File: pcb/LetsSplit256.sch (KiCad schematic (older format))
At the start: 62 parts, among them J1 AudioJack3_Ground, U1 ProMicro

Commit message: Add footprints for switch and pro micro
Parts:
- DL11, DL12, DL13, DL14, DL15, DL21, DL22, DL23, DL24, DL25, DL31, DL32, DL33, DL34, DL35, DL41, DL42, DL43, DL44, DL45, DL51, DL52, DL53, DL54, DL55, DL61, DL62, DL63, DL64, DL65: footprint Diodes_THT:D_DO-35_SOD27_P7.62mm_Horizontal -> Diode_THT:D_DO-35_SOD27_P7.62mm_Horizontal
- KL1, KL2, KL3, KL4, KL5, KLA1, KLB1, KLC1, KLD1, KLE1, KLF1, KLFunc11, KLFunc12, KLFunc13, KLFunc14, KLFunc15, KLFunc25, KLFunc35, KLFunc45, KLFunc55, KLFunc65, KLG1, KLQ1, KLR1, KLS1, KLT1, KLV1, KLW1, KLX1, KLZ1: footprint Button_Switch_Keyboard:SW_Cherry_MX1A_1.00u_Plate -> pcb:cherry
- U1: footprint promicro:ProMicro -> pcb:ProMicro

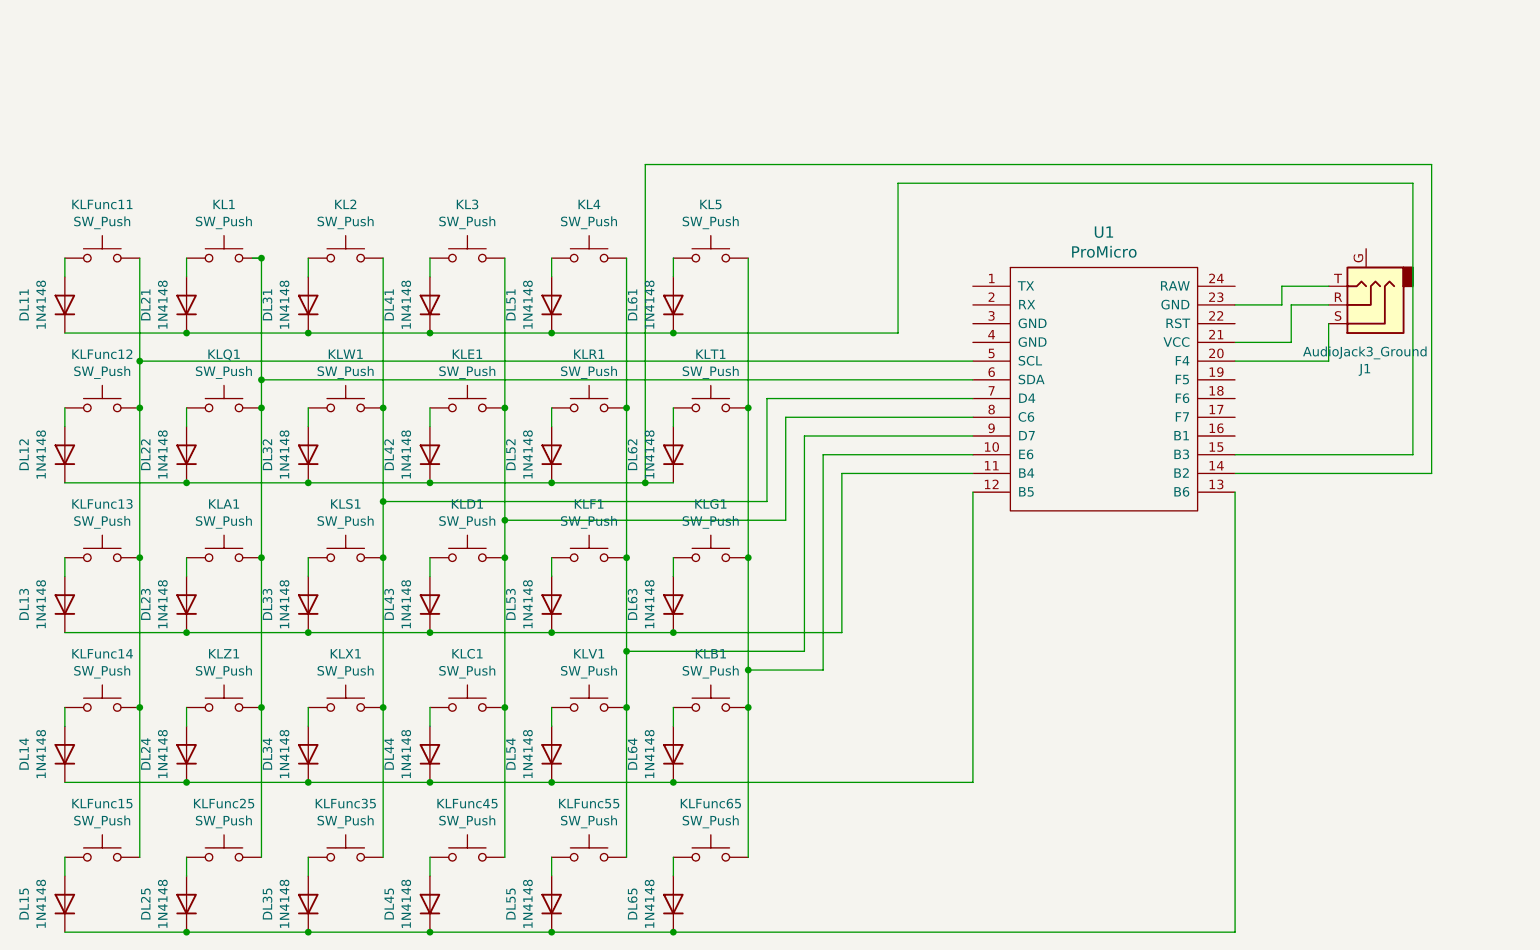
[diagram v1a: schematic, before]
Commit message: Routing
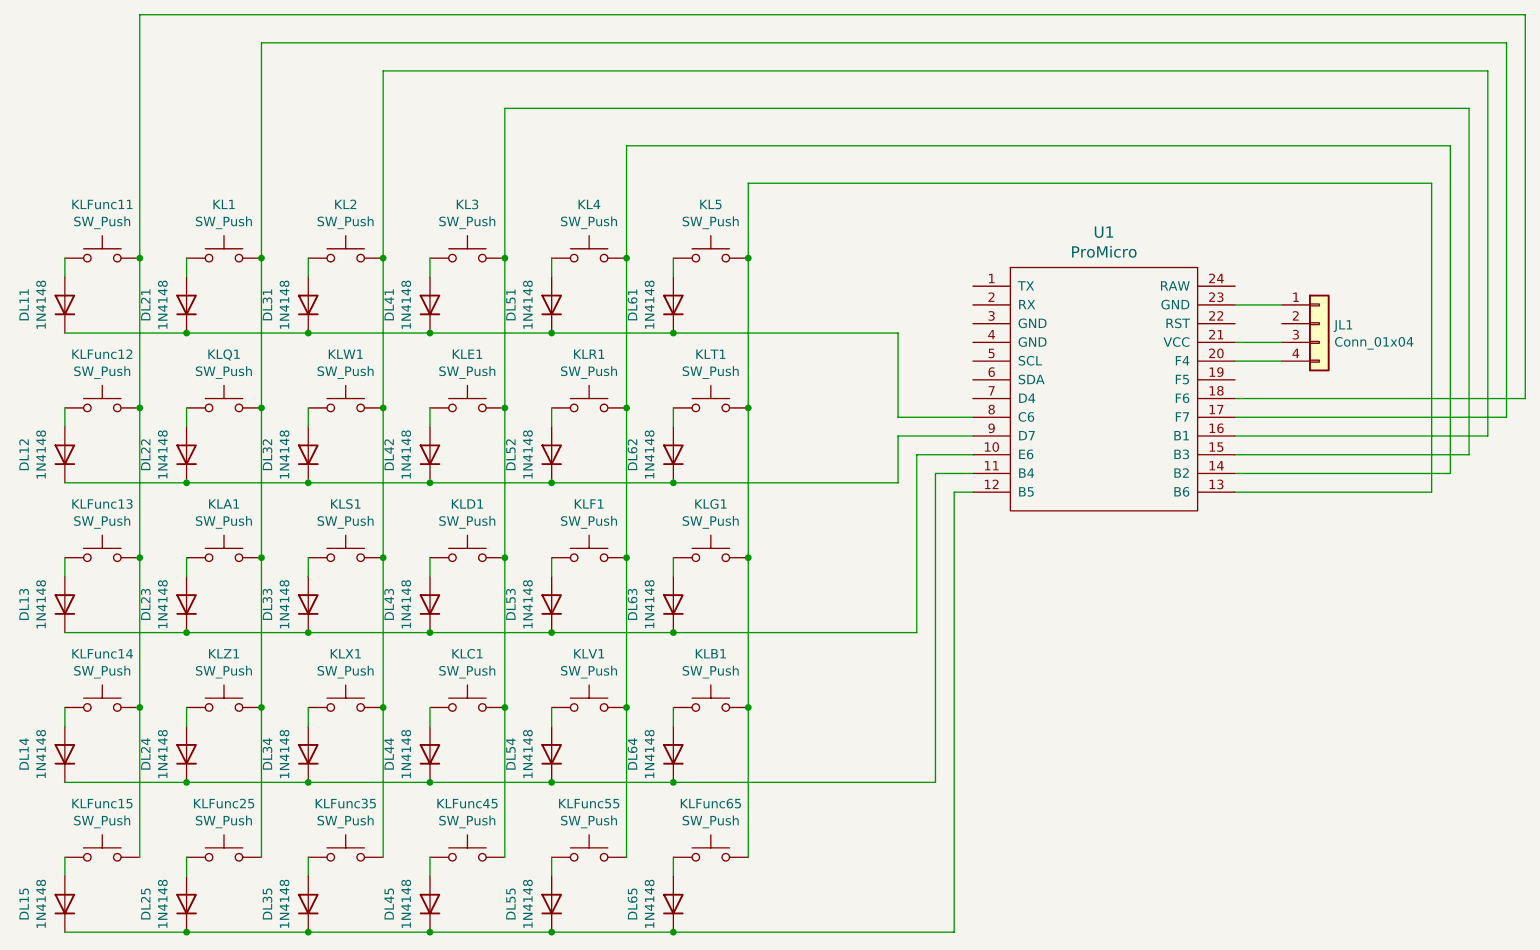
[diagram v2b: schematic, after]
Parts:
- removed J1: AudioJack3_Ground, xess:PJ-313-TH_mod, symbol Connector:AudioJack3_Ground
- added JL1: Conn_01x04, Connector_PinHeader_2.54mm:PinHeader_1x04_P2.54mm_Horizontal, symbol Connector_Generic:Conn_01x04
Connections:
- net at KL5.2, KLB1.2, KLFunc65.2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: now also U1.13 (B6); no longer U1.10 (E6)
- net at DL13.1 (K), DL23.1 (K), DL33.1 (K)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: now also U1.10 (E6); no longer U1.11 (B4)
- net at DL14.1 (K), DL24.1 (K), DL34.1 (K)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: now also U1.11 (B4); no longer U1.12 (B5)
- net at DL15.1 (K), DL25.1 (K), DL35.1 (K)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: now also U1.12 (B5); no longer U1.13 (B6)
- net at DL12.1 (K), DL22.1 (K), DL32.1 (K)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: now also U1.9 (D7); no longer U1.14 (B2)
- net at DL11.1 (K), DL21.1 (K), DL31.1 (K)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: now also U1.8 (C6); no longer U1.15 (B3)
- net at U1.16 (B1): now also KL2.2, KLFunc35.2, KLS1.2, KLW1.2, KLX1.2
- net at U1.17 (F7): now also KL1.2, KLA1.2, KLFunc25.2, KLQ1.2, KLZ1.2
- net at U1.18 (F6): now also KLFunc11.2, KLFunc12.2, KLFunc13.2, KLFunc14.2, KLFunc15.2
- net at U1.20 (F4): now also JL1.4 (Pin_4)
- net at U1.21 (VCC): now also JL1.3 (Pin_3)
- net at U1.23 (GND): now also JL1.1 (Pin_1)
- net at KL3.2, KLC1.2, KLD1.2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: now also U1.15 (B3); no longer U1.8 (C6)
- net at KL4.2, KLF1.2, KLFunc55.2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: now also U1.14 (B2); no longer U1.9 (D7)
- now unconnected: U1.5 (SCL), U1.6 (SDA), U1.7 (D4)
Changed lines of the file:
@@
 	3700 3800 4350 3800
 Connection ~ 3700 3800
-Wire Wire Line
-	4350 3800 4850 3800
 Connection ~ 4350 3800
 Wire Wire Line
@@
 	2150 4200 2150 5000
 Connection ~ 2150 4200
-Wire Wire Line
-	2800 2600 2800 3250
-Connection ~ 2800 3400
 Wire Wire Line
 	2800 4200 2800 5000
@@
 	5400 3400 5400 4200
 Connection ~ 5400 3400
-Wire Wire Line
-	5400 4200 5400 4800
 Connection ~ 5400 4200
-$Comp
-L Connector:AudioJack3_Ground J1
-U 1 1 5BBB5B1E
-P 8700 2850
-F 0 "J1" H 8704 3192 50  0000 C CNN
-F 1 "AudioJack3_Ground" H 8704 3101 50  0000 C CNN
-F 2 "xess:PJ-313-TH_mod" H 8700 2850 50  0001 C CNN
-F 3 "~" H 8700 2850 50  0001 C CNN
-	1    8700 2850
-	-1   0    0    1
-$EndComp
-Wire Wire Line
-	4100 3400 4100 4000
 Wire Wire Line
 	3450 4200 3450 5000
@@
 Wire Wire Line
 	2150 3400 2150 4200
-Connection ~ 2800 2600
-Wire Wire Line
-	2800 2600 2750 2600
 Wire Wire Line
 	4100 4200 4100 5000
-Wire Wire Line
-	4750 4200 4750 4700
-Wire Wire Line
-	3450 3400 3450 3900
-Wire Wire Line
-	6600 3250 2800 3250
-Connection ~ 2800 3250
-Wire Wire Line
-	2800 3250 2800 3400
-Wire Wire Line
-	2150 2600 2150 3150
-Wire Wire Line
-	6600 3150 2150 3150
-Connection ~ 2150 3150
-Wire Wire Line
-	2150 3150 2150 3400
-Wire Wire Line
-	6600 3350 5500 3350
-Wire Wire Line
-	5500 3350 5500 3900
-Wire Wire Line
-	5500 3900 3450 3900
-Connection ~ 3450 3900
-Wire Wire Line
-	3450 3900 3450 4200
-Wire Wire Line
-	6600 3450 5600 3450
-Wire Wire Line
-	5600 3450 5600 4000
-Wire Wire Line
-	5600 4000 4100 4000
-Connection ~ 4100 4000
-Wire Wire Line
-	4100 4000 4100 4200
-Wire Wire Line
-	6600 3550 5700 3550
-Wire Wire Line
-	5700 3550 5700 4700
-Wire Wire Line
-	5700 4700 4750 4700
-Connection ~ 4750 4700
-Wire Wire Line
-	4750 4700 4750 5000
-Wire Wire Line
-	5400 4800 5800 4800
-Wire Wire Line
-	5800 4800 5800 3650
-Wire Wire Line
-	5800 3650 6600 3650
-Connection ~ 5400 4800
-Wire Wire Line
-	5400 4800 5400 5000
-Wire Wire Line
-	5000 5400 6600 5400
-Wire Wire Line
-	6600 5400 6600 3850
-Connection ~ 5000 5400
-Wire Wire Line
-	6600 3750 5900 3750
-Wire Wire Line
-	5900 3750 5900 4600
-Wire Wire Line
-	5900 4600 5000 4600
-Connection ~ 5000 4600
-Wire Wire Line
-	4850 2100 4850 3800
-Connection ~ 4850 3800
-Wire Wire Line
-	4850 3800 5000 3800
-Wire Wire Line
-	5000 3000 6200 3000
-Wire Wire Line
-	6200 3000 6200 2200
-Wire Wire Line
-	6200 2200 8950 2200
-Wire Wire Line
-	8950 2200 8950 3650
-Wire Wire Line
-	8950 3650 8000 3650
-Connection ~ 5000 3000
-Wire Wire Line
-	9050 2100 9050 3750
-Wire Wire Line
-	9050 3750 8000 3750
-Wire Wire Line
-	4850 2100 9050 2100
-Wire Wire Line
-	8500 2750 8250 2750
-Wire Wire Line
-	8250 2750 8250 2850
-Wire Wire Line
-	8250 2850 8000 2850
-Wire Wire Line
-	8500 2850 8300 2850
-Wire Wire Line
-	8300 2850 8300 3050
-Wire Wire Line
-	8300 3050 8000 3050
-Wire Wire Line
-	8000 3150 8500 3150
-Wire Wire Line
-	8500 3150 8500 2950
 Connection ~ 5400 5000
 Connection ~ 4750 5000
@@
 	1750 6200 2400 6200
 Connection ~ 2400 6200
-Wire Wire Line
-	5000 6200 8000 6200
-Wire Wire Line
-	8000 3850 8000 6200
-Connection ~ 5000 6200
 $Comp
 L Diode:1N4148 DL11
@@
 	1    0    0    -1
 $EndComp
+$Comp
+L Connector_Generic:Conn_01x04 JL1
+U 1 1 605629C9
+P 8450 2950
+F 0 "JL1" H 8530 2942 50  0000 L CNN
+F 1 "Conn_01x04" H 8530 2851 50  0000 L CNN
+F 2 "Connector_PinHeader_2.54mm:PinHeader_1x04_P2.54mm_Horizontal" H 8450 2950 50  0001 C CNN
+F 3 "~" H 8450 2950 50  0001 C CNN
+	1    8450 2950
+	1    0    0    -1
+$EndComp
+Wire Wire Line
+	4750 4200 4750 5000
+Wire Wire Line
+	5400 4200 5400 5000
+Wire Wire Line
+	2150 2600 2150 3400
+Wire Wire Line
+	3450 3400 3450 4200
+Wire Wire Line
+	4100 3400 4100 4200
+Wire Wire Line
+	4350 3800 5000 3800
+Wire Wire Line
+	8000 2850 8250 2850
+Wire Wire Line
+	8000 3150 8250 3150
+Wire Wire Line
+	8000 3050 8250 3050
+Connection ~ 4750 2600
+Wire Wire Line
+	5400 2600 5400 2200
+Wire Wire Line
+	5400 2200 9050 2200
+Connection ~ 5400 2600
+Wire Wire Line
+	4750 2000 9150 2000
+Wire Wire Line
+	4750 2000 4750 2600
+Wire Wire Line
+	4100 2600 4100 1800
+Wire Wire Line
+	4100 1800 9250 1800
+Connection ~ 4100 2600
+Wire Wire Line
+	9350 1600 3450 1600
+Wire Wire Line
+	3450 1600 3450 2600
+Connection ~ 3450 2600
+Wire Wire Line
+	2800 2600 2800 3400
+Connection ~ 2800 3400
+Wire Wire Line
+	2800 2600 2800 1450
+Wire Wire Line
+	2800 1450 9450 1450
+Wire Wire Line
+	9450 1450 9450 3450
+Connection ~ 2800 2600
+Wire Wire Line
+	9550 1300 2150 1300
+Wire Wire Line
+	2150 1300 2150 2600
+Connection ~ 2150 2600
+Wire Wire Line
+	5000 3000 6200 3000
+Wire Wire Line
+	6200 3000 6200 3450
+Wire Wire Line
+	6200 3450 6600 3450
+Connection ~ 5000 3000
+Wire Wire Line
+	5000 3800 6200 3800
+Wire Wire Line
+	6200 3800 6200 3550
+Wire Wire Line
+	6200 3550 6600 3550
+Connection ~ 5000 3800
+Wire Wire Line
+	6600 3650 6300 3650
+Wire Wire Line
+	6300 3650 6300 4600
+Wire Wire Line
+	6300 4600 5000 4600
+Connection ~ 5000 4600
+Wire Wire Line
+	5000 5400 6400 5400
+Wire Wire Line
+	6400 5400 6400 3750
+Wire Wire Line
+	6400 3750 6600 3750
+Connection ~ 5000 5400
+Wire Wire Line
+	6600 3850 6500 3850
+Wire Wire Line
+	6500 3850 6500 6200
+Wire Wire Line
+	6500 6200 5000 6200
+Connection ~ 5000 6200
+Wire Wire Line
+	9050 3850 8000 3850
+Wire Wire Line
+	9050 2200 9050 3850
+Wire Wire Line
+	8000 3750 9150 3750
+Wire Wire Line
+	9150 2000 9150 3750
+Wire Wire Line
+	9250 3650 8000 3650
+Wire Wire Line
+	9250 1800 9250 3650
+Wire Wire Line
+	8000 3550 9350 3550
+Wire Wire Line
+	9350 3550 9350 1600
+Wire Wire Line
+	8000 3450 9450 3450
+Wire Wire Line
+	8000 3350 9550 3350
+Wire Wire Line
+	9550 3350 9550 1300
 $EndSCHEMATC
